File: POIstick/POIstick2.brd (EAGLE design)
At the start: 98.7 x 22.9 mm, 43 parts, among them SW1 431151015826, SW2 431151015826, U1 CR2032-SNAPDRAGONCR2032, X1 2MHz

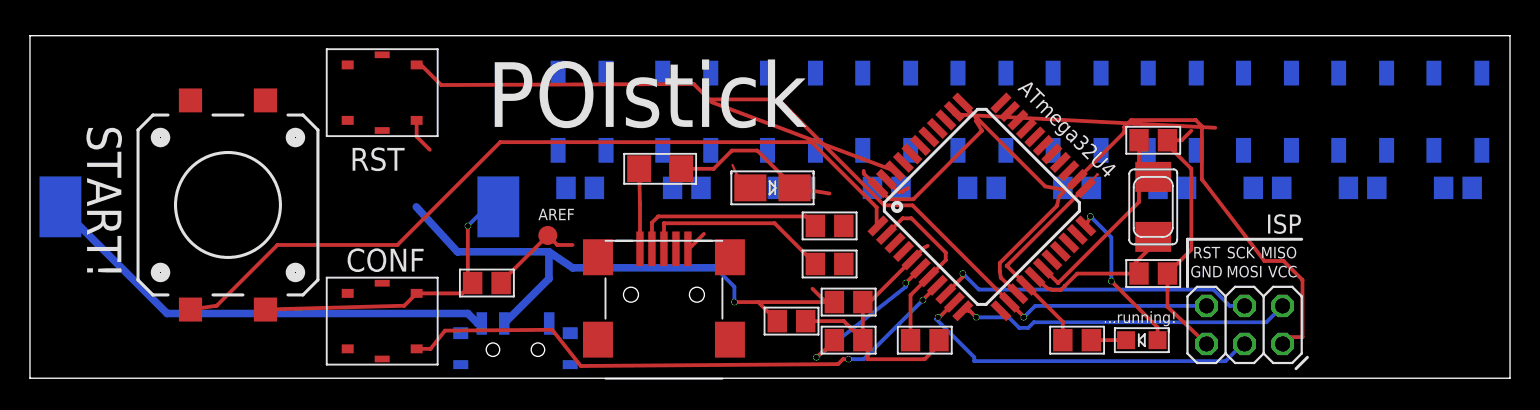
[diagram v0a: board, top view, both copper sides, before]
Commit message: WIP
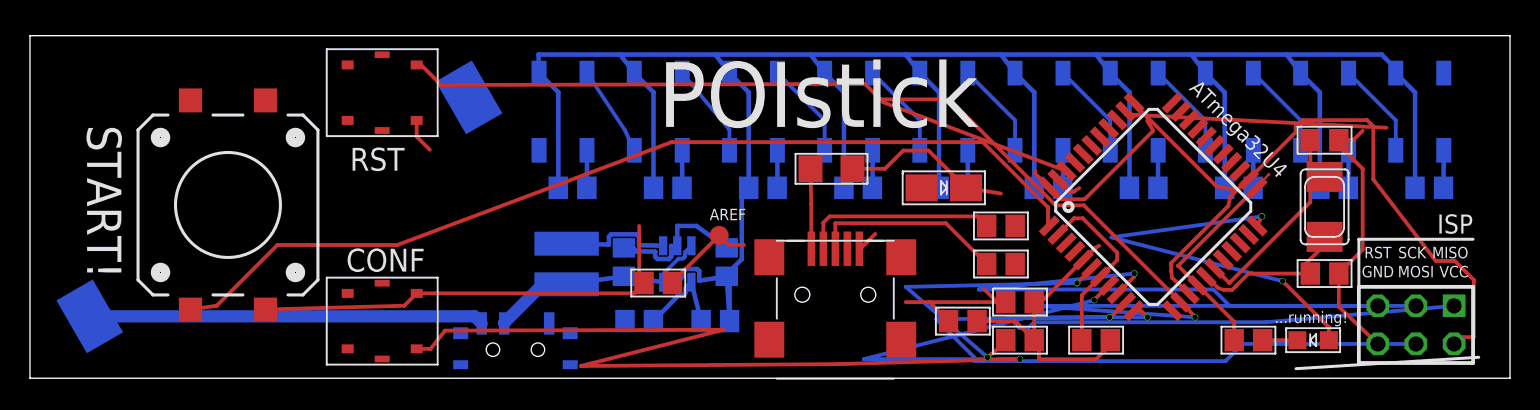
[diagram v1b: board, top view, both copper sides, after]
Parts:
- added C19: 4.7uF, microbuilder:0805
- added C20: 10uF, microbuilder:0805
- added L1: 4.7uH, WE-TPC:WE-TPC_3816
- added R3: 976K, microbuilder:0805
- added R4: 309K, microbuilder:0805
- added U$2: MCP1623/24, MCP1623:SOT95P300X120-6N
- X1: value 2MHz -> 8MHz
- moved C3 11.4 mm to (76.2, 22.9)
- moved C5 11.4 mm to (81.3, 20.3)
- moved C6 11.4 mm to (71.1, 30.5)
- moved C8 11.4 mm to (76.2, 20.3)
- moved R1 11.4 mm to (74.9, 25.4)
- moved R2 11.4 mm to (74.9, 27.9)
- moved U$1 11.4 mm to (85.1, 29.2)
- moved AREF 11.4 mm to (56.1, 27.3)
- moved C4 11.4 mm to (72.4, 21.6)
- moved C7 11.4 mm to (52.1, 24.1)
- moved CN1 11.4 mm to (63.9, 22.4)
- moved PTCFUSE 11.4 mm to (63.6, 31.8)
- moved C1 11.4 mm to (96.5, 33.7)
- moved C2 11.4 mm to (96.5, 24.8)
- moved ISP 11.4 mm to (102.6, 21.3)
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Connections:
- removed net N$18: R1.2
- removed net N$4: U$1.4
- new net USB_D+: R1.2, U$1.4
- new net USB_D-: R2.2, U$1.3
- new net VIN: C19.1, L1.1, S3.2, U$2.3, U$2.6
- net GND: now also C19.2, C20.2, R4.2, U$2.2
- net N$19: now also L1.2, U$2.1; no longer R2.2
- net N$3: now also R3.2, R4.1, U$2.4; no longer U$1.3
- net VCC: now also C20.1, R3.1, U$2.5; no longer S3.2
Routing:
- net VCC: track 101.0 -> 240.9 mm, vias 1 -> 0
- net PB0: track 38.7 -> 87.9 mm
- net GND: track 98.9 -> 140.8 mm, vias 1 -> 0
- net RST: track 60.4 -> 92.9 mm
- net MOSI: track 24.0 -> 46.8 mm
- net SCK: track 21.5 -> 41.9 mm
- net MISO: track 22.4 -> 40.5 mm
- net PD5: track 10.8 -> 27.8 mm
- net VIN: track 0.00 -> 15.2 mm
- net N$34: track 11.0 -> 21.8 mm
- net PE6: track 53.4 -> 63.2 mm
- net N$19: track 0.00 -> 7.68 mm
- net N$3: track 0.00 -> 6.48 mm
- net N$15: track 0.00 -> 6.46 mm
- net N$13: track 0.00 -> 6.46 mm
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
